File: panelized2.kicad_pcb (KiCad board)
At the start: 2 copper layers, 74.9 x 98 mm, 134 parts, among them J1 Conn_01x05_Male, J2 Conn_01x02_Male, J3 Conn_01x08_Male, J4 Conn_01x02_Male, J5 Conn_01x02_Male, J6 Conn_01x06_Male, J7 Conn_01x02_Male, U1 NCP1117ST33T3G, U2 STM32F042G6Ux, U3 SN65HVD233, Y1 Crystal_GND24

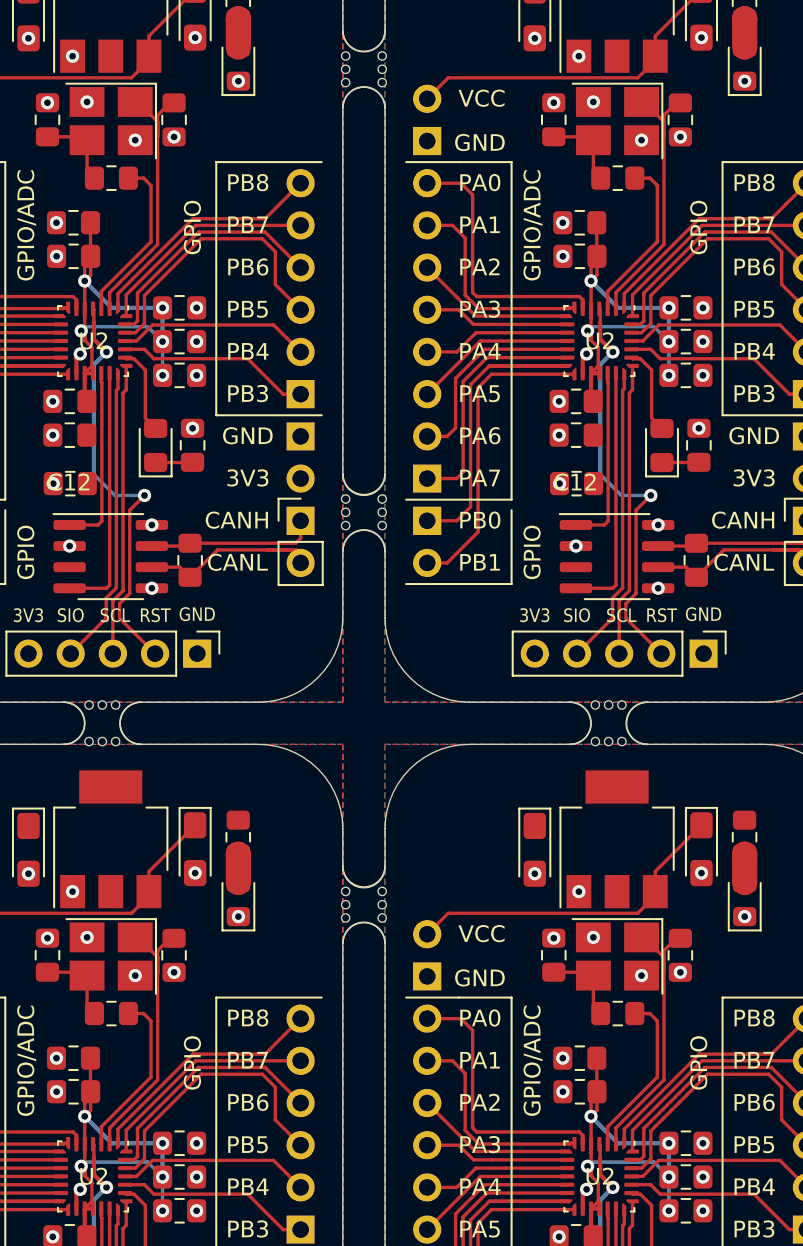
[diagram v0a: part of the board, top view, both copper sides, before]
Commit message: pcb smt assembly
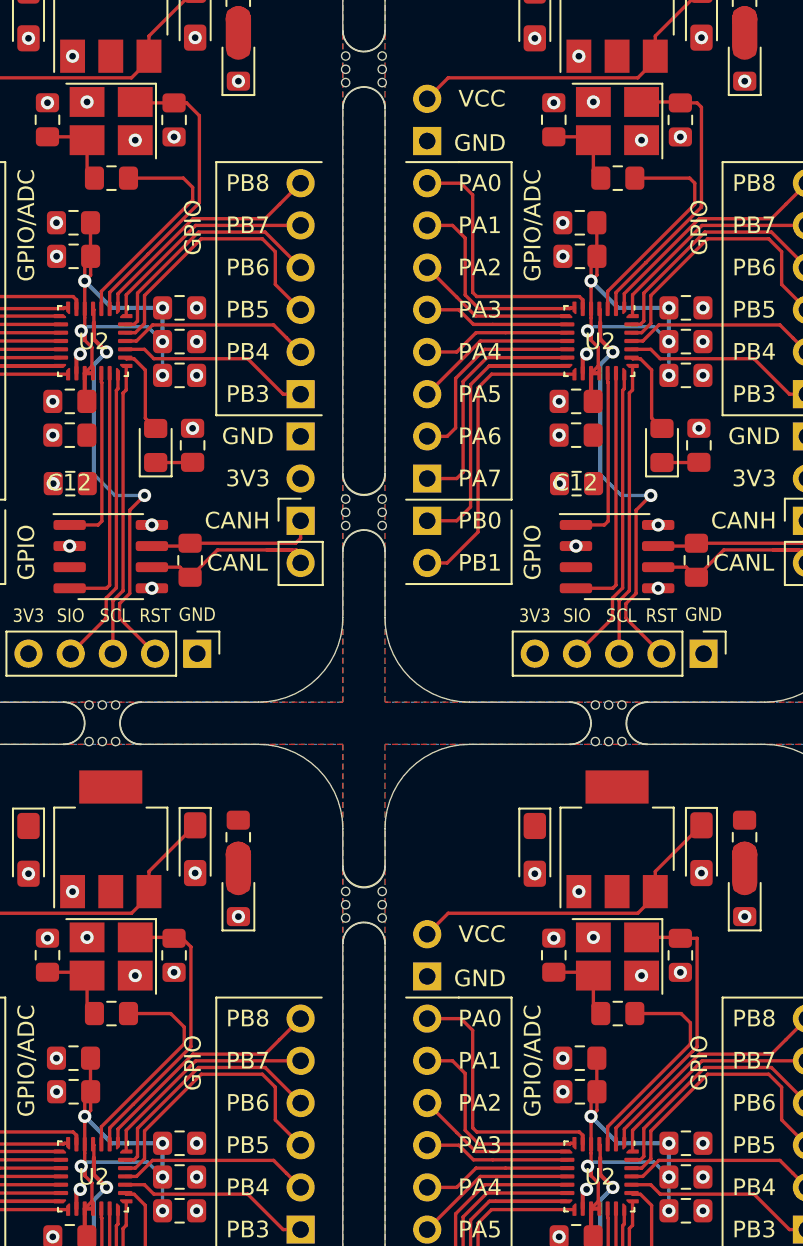
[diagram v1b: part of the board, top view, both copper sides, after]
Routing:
- net /OSC_N: track 40.8 -> 52.9 mm
- net /OSC_P: track 67.0 -> 71.8 mm
